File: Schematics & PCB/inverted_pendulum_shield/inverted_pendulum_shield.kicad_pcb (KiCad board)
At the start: 2 copper layers, 76 x 72 mm, 48 parts, among them J1 Screw_Terminal_01x02, J2 Screw_Terminal_01x04, J3 Screw_Terminal_01x02, J4 FCR7350R, J5 FCR7350B, Q1 DMP3056L-7, Q2 NX138BKR, Q3 FQD8P10TM, Q4 SLMT320V3CN, Q5 SLMT320V3CN, SW1 1825027, U1 DRV8231DDAR, U2 AP63301WU-7

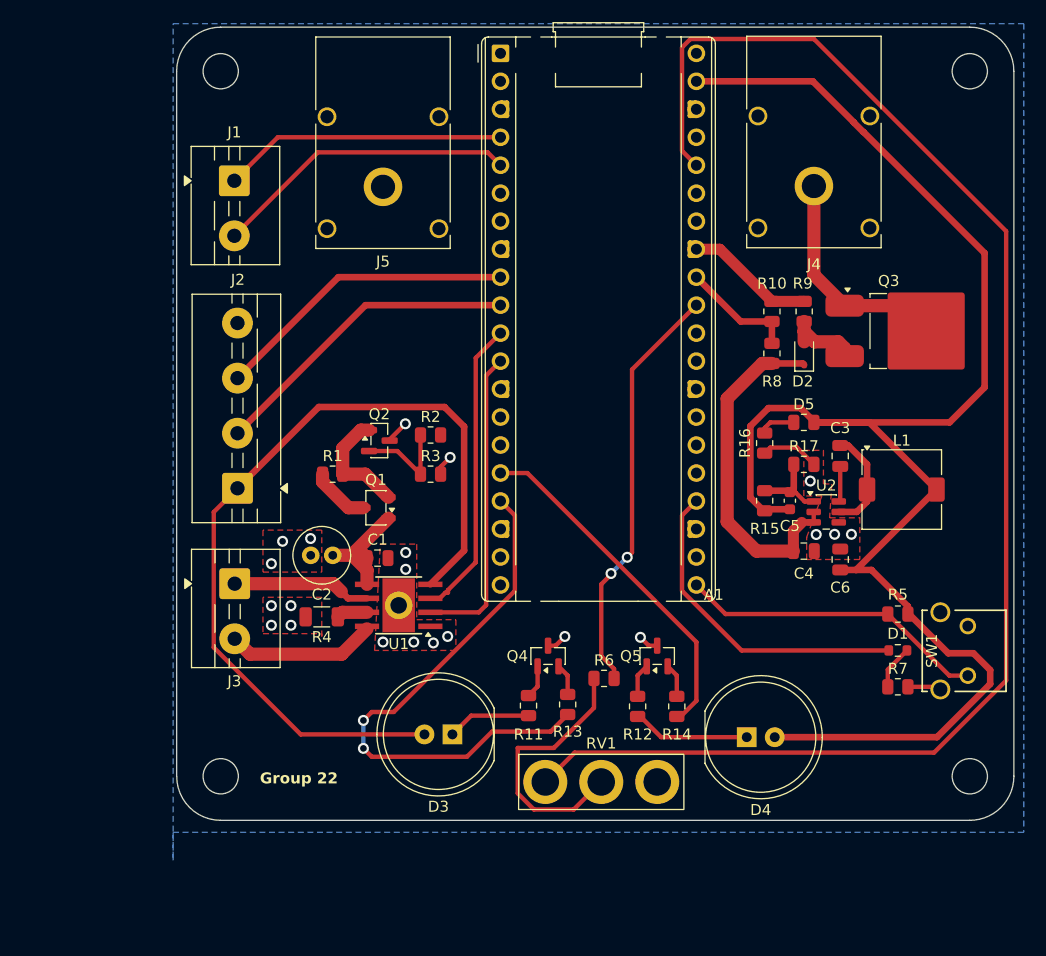
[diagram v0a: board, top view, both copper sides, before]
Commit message: finished revision 2 of pcb and schematics
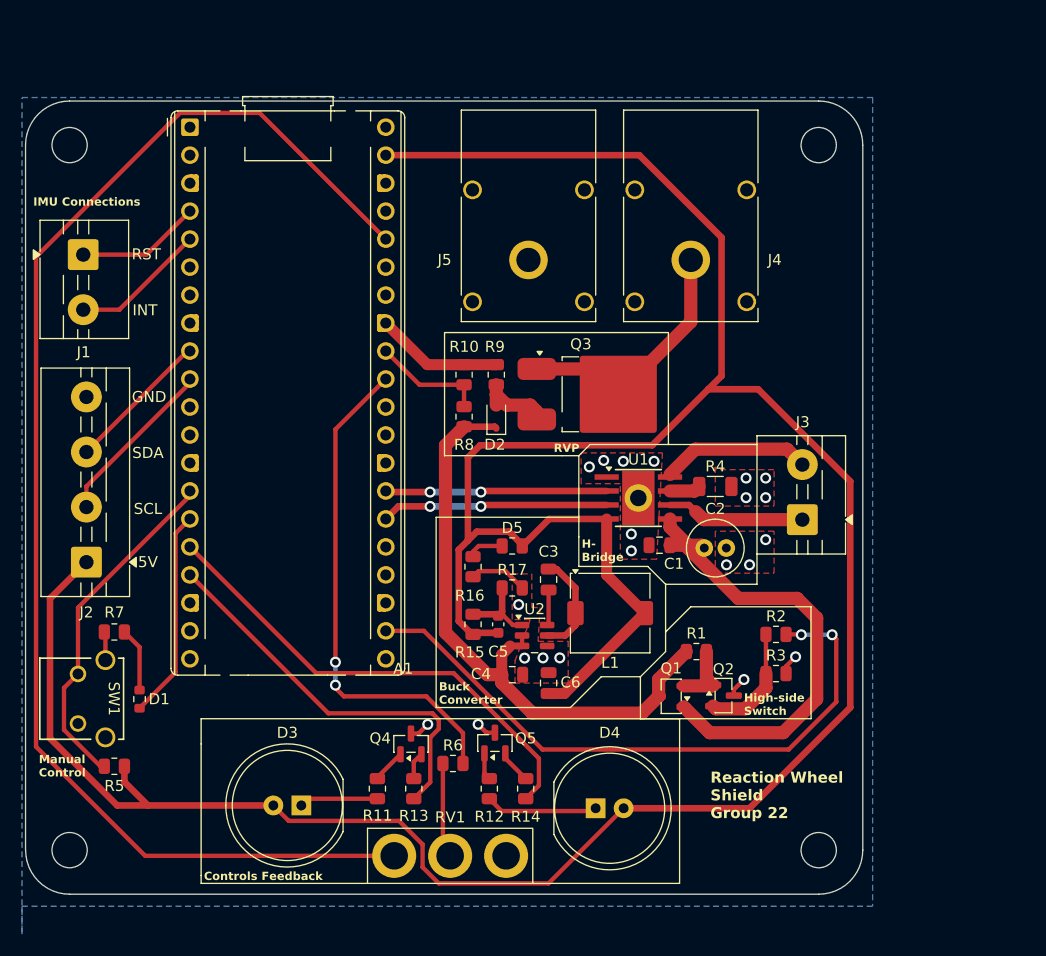
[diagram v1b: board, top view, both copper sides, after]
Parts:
- moved SW1 80.8 mm to (111.0, 121.8), turned to -90 degrees
- moved R5 72.4 mm to (114.3, 130.1)
- moved R7 71.3 mm to (114.3, 118.0), turned to 180 degrees
- moved D1 69.0 mm to (116.6, 124.1), turned to -90 degrees
- moved J3 51.9 mm to (176.8, 107.8), turned to 90 degrees
- moved Q2 38.9 mm to (169.6, 123.7)
- moved R4 37.6 mm to (168.8, 104.7), turned to 0 degrees
- moved R1 36.7 mm to (167.1, 119.7)
- moved R2 36.2 mm to (174.4, 118.2)
- moved R3 36.2 mm to (174.4, 121.7)
- moved C2 33.7 mm to (167.8, 110.3), turned to 0 degrees
- moved Q1 31.8 mm to (164.8, 123.8)
- moved A1 29.0 mm to (121.2, 72.1)
- moved L1 28.8 mm to (159.3, 116.2)
- moved R16 28.8 mm to (146.9, 112.0)
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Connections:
- A1 pad 11: Motor Control 1 -> unconnected-(A1-GPIO8-Pad11)
- A1 pad 12: Motor Control 2 -> unconnected-(A1-GPIO9-Pad12)
- A1 pad 14: unconnected-(A1-GPIO10-Pad14) -> Controls Start
- A1 pad 15: unconnected-(A1-GPIO11-Pad15) -> /LED_indicate
- A1 pad 21: Controls Start -> unconnected-(A1-GPIO16-Pad21)
- A1 pad 24: /LED_indicate -> unconnected-(A1-GPIO18-Pad24)
- A1 pad 26: unconnected-(A1-GPIO20-Pad26) -> Motor Control 1
- A1 pad 27: unconnected-(A1-GPIO21-Pad27) -> Motor Control 2
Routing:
- net Motor_SW: track 0.00 -> 57.6 mm, vias 0 -> 2
- net +5V: track 221.6 -> 272.5 mm
- net Net-(Q1-D): track 11.0 -> 42.5 mm
- net Vin: track 36.7 -> 55.6 mm
- net Net-(R6-Pad1): track 24.4 -> 8.65 mm
- net IMU_INT: track 27.8 -> 12.3 mm
- net IMU_RST: track 25.8 -> 11.3 mm
- net IMU_SDA: track 27.7 -> 13.2 mm
- net LED_PWM_1: track 50.3 -> 36.1 mm, vias 2 -> 0
- net IMU_SCL: track 28.7 -> 15.5 mm
- net LED_PWM_2: track 31.8 -> 43.8 mm
- net +3.3V: track 134.6 -> 123.0 mm
- net /LED_indicate: track 29.7 -> 19.1 mm
- net ADC0: track 37.9 -> 46.0 mm
- net Motor Control 2: track 28.0 -> 20.1 mm, vias 0 -> 2
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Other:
- board text added: "5V"
- board text added: "Buck Converter"
- board text added: "Controls Feedback"
- board text added: "GND"
- board text added: "H- Bridge"
- board text added: "High-side Switch"
- board text added: "IMU Connections"
- board text added: "INT"
- board text added: "Manual Control"
- board text added: "RST"
- board text added: "RVP"
- board text added: "Reaction Wheel Shield Group 22"
- board text added: "SCL"
- board text added: "SDA"
- board text removed: "Group 22"
